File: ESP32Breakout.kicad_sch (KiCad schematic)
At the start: 5 parts, among them J1 PIN6-9_Breakout, J2 PIN10-13_Breakout, U1 ESP32-S3

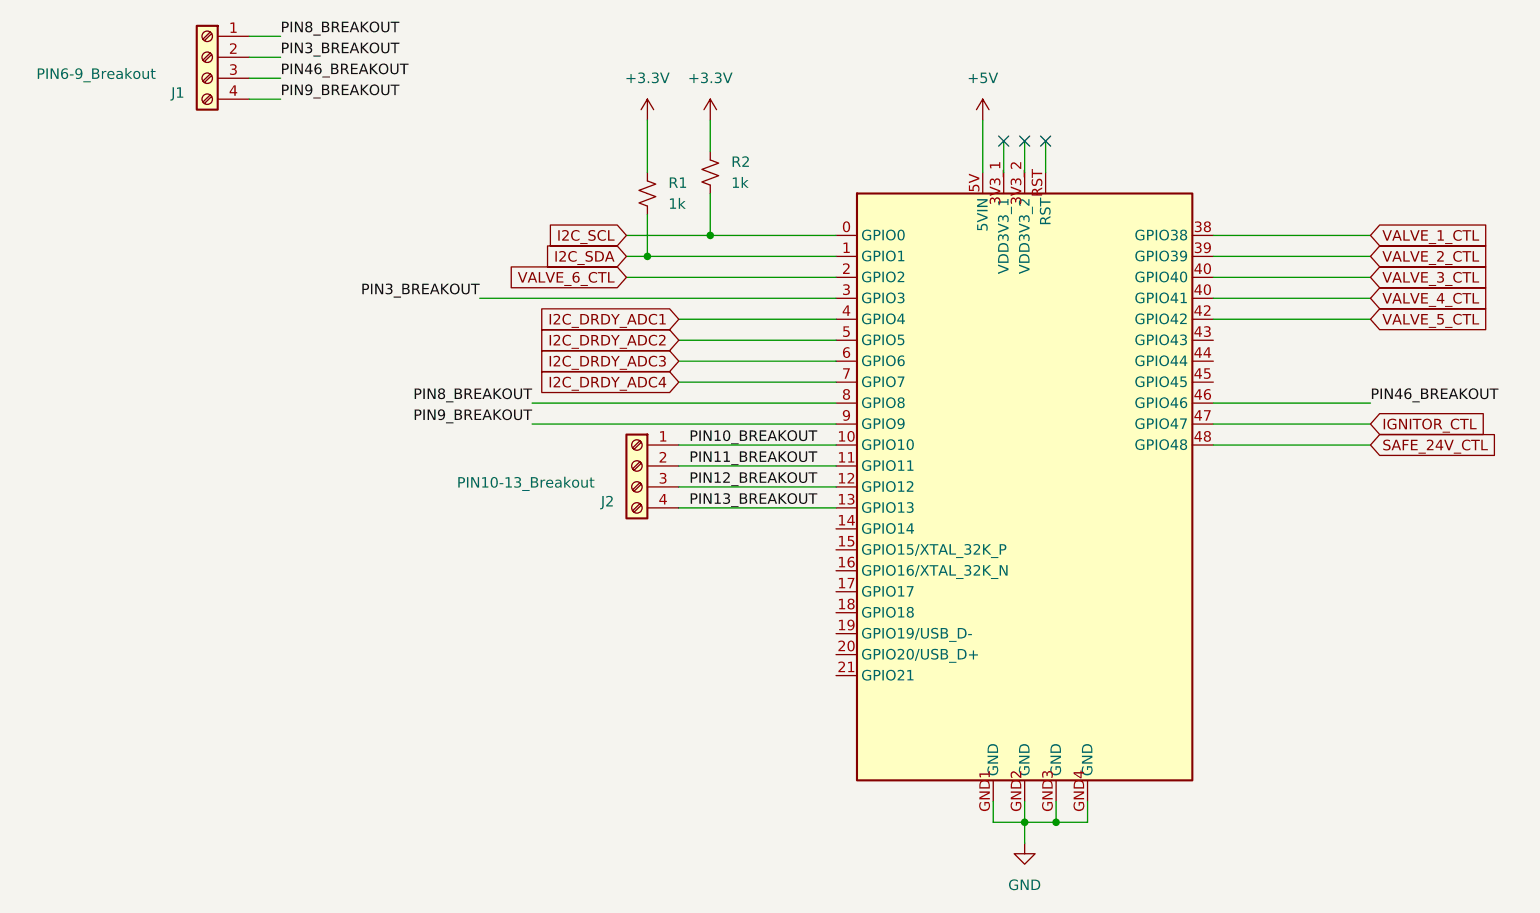
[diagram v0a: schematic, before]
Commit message: Satisfy DRC
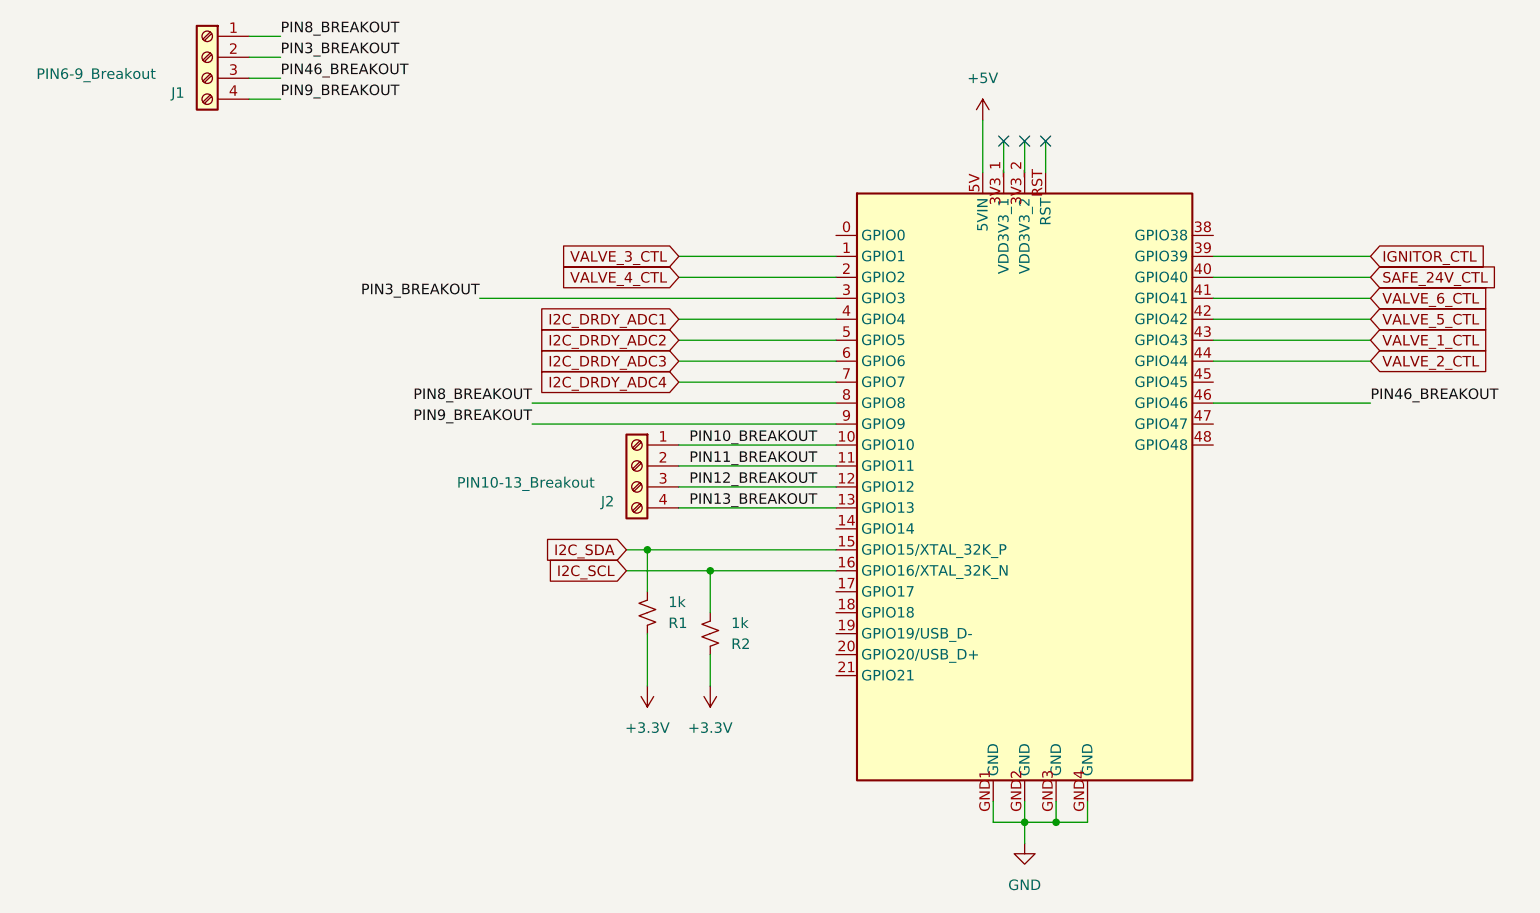
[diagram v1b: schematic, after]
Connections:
- net I2C_SCL: now also U1.16 (GPIO16/XTAL_32K_N); no longer U1.0 (GPIO0)
- net I2C_SDA: now also U1.15 (GPIO15/XTAL_32K_P); no longer U1.1 (GPIO1)
- net IGNITOR_CTL: now also U1.39 (GPIO39); no longer U1.47 (GPIO47)
- net SAFE_24V_CTL: now also U1.40 (GPIO40); no longer U1.48 (GPIO48)
- net VALVE_1_CTL: now also U1.43 (GPIO43); no longer U1.38 (GPIO38)
- net VALVE_2_CTL: now also U1.44 (GPIO44); no longer U1.39 (GPIO39)
- net VALVE_3_CTL: now also U1.1 (GPIO1); no longer U1.40 (GPIO41)
- net VALVE_4_CTL: now also U1.2 (GPIO2); no longer U1.40 (GPIO41)
- net VALVE_6_CTL: now also U1.41 (GPIO41); no longer U1.2 (GPIO2)
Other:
- moved on the sheet: R1, R2
